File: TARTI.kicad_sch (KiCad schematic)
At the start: 7 parts, among them J1 Conn_01x04_Socket, J2 Conn_01x04_Socket, J3 Screw_Terminal_01x02, U1 LM7805_TO220

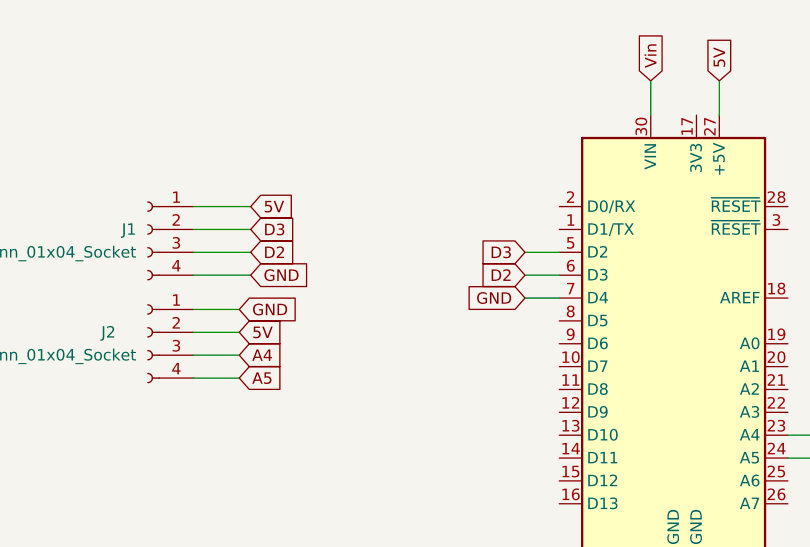
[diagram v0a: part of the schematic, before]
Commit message: Add files via upload
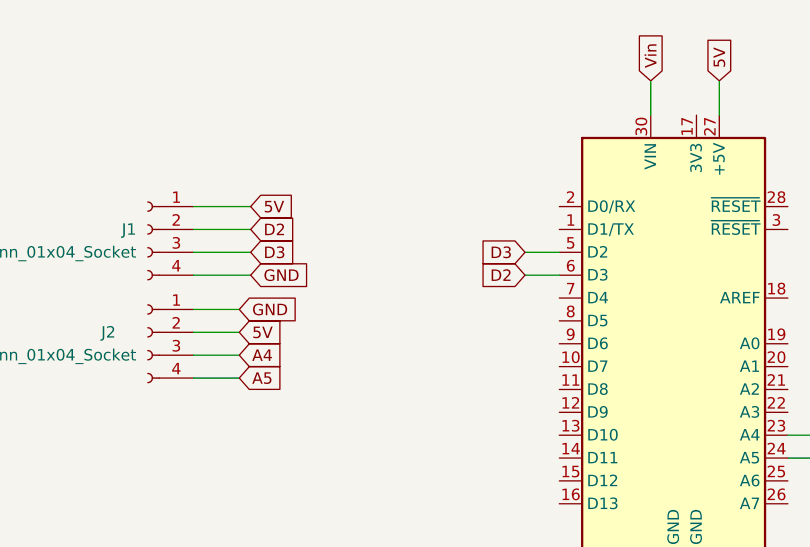
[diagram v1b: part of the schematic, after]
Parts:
- J1, J2: footprint Connector_PinHeader_1.27mm:PinHeader_1x04_P1.27mm_Vertical -> Connector_PinSocket_2.54mm:PinSocket_1x04_P2.54mm_Vertical
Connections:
- net D2: now also J1.2 (Pin_2); no longer J1.3 (Pin_3)
- net D3: now also J1.3 (Pin_3); no longer J1.2 (Pin_2)
- net GND: no longer A1.7 (D4)
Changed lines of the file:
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@@
-		)
-	)
-	(wire
-		(pts
-			(xy 106.68 63.5) (xy 110.49 63.5)
-		)
-		(stroke
-			(width 0)
-			(type default)
 		)
 	)
@@
 		)
 	)
+	(global_label "D2"
+		(shape input)
+		(at 76.2 55.88 0)
+		(fields_autoplaced yes)
+		(effects
+			(font
+				(size 1.27 1.27)
+			)
+			(justify left)
+		)
+		(property "Intersheetrefs" "${INTERSHEET_REFS}"
+			(at 81.6647 55.88 0)
+			(effects
+				(font
+					(size 1.27 1.27)
+				)
+				(justify left)
+				(hide yes)
+			)
+		)
+	)
+	(global_label "GND"
+		(shape input)
+		(at 123.19 97.79 270)
+		(fields_autoplaced yes)
+		(effects
+			(font
+				(size 1.27 1.27)
+			)
+			(justify right)
+		)
+		(property "Intersheetrefs" "${INTERSHEET_REFS}"
+			(at 123.19 104.6457 90)
+			(effects
+				(font
+					(size 1.27 1.27)
+				)
+				(justify right)
+				(hide yes)
+			)
+		)
+	)
+	(global_label "GND"
+		(shape input)
+		(at 49.53 138.43 180)
+		(fields_autoplaced yes)
+		(effects
+			(font
+				(size 1.27 1.27)
+			)
+			(justify right)
+		)
+		(property "Intersheetrefs" "${INTERSHEET_REFS}"
+			(at 42.6743 138.43 0)
+			(effects
+				(font
+					(size 1.27 1.27)
+				)
+				(justify right)
+				(hide yes)
+			)
+		)
+	)
+	(global_label "Vin"
+		(shape input)
+		(at 120.65 39.37 90)
+		(fields_autoplaced yes)
+		(effects
+			(font
+				(size 1.27 1.27)
+			)
+			(justify left)
+		)
+		(property "Intersheetrefs" "${INTERSHEET_REFS}"
+			(at 120.65 33.5424 90)
+			(effects
+				(font
+					(size 1.27 1.27)
+				)
+				(justify left)
+				(hide yes)
+			)
+		)
+	)
 	(global_label "D3"
 		(shape input)
-		(at 76.2 55.88 0)
-		(fields_autoplaced yes)
-		(effects
-			(font
-				(size 1.27 1.27)
-			)
-			(justify left)
-		)
-		(property "Intersheetrefs" "${INTERSHEET_REFS}"
-			(at 81.6647 55.88 0)
-			(effects
-				(font
-					(size 1.27 1.27)
-				)
-				(justify left)
-				(hide yes)
-			)
-		)
-	)
-	(global_label "GND"
-		(shape input)
-		(at 123.19 97.79 270)
+		(at 76.2 58.42 0)
+		(fields_autoplaced yes)
+		(effects
+			(font
+				(size 1.27 1.27)
+			)
+			(justify left)
+		)
+		(property "Intersheetrefs" "${INTERSHEET_REFS}"
+			(at 81.6647 58.42 0)
+			(effects
+				(font
+					(size 1.27 1.27)
+				)
+				(justify left)
+				(hide yes)
+			)
+		)
+	)
+	(global_label "D3"
+		(shape input)
+		(at 106.68 58.42 180)
 		(fields_autoplaced yes)
 		(effects
@@
 		)
 		(property "Intersheetrefs" "${INTERSHEET_REFS}"
-			(at 123.19 104.6457 90)
+			(at 101.2153 58.42 0)
 			(effects
 				(font
@@
 		)
 	)
-	(global_label "GND"
-		(shape input)
-		(at 49.53 138.43 180)
+	(global_label "A5"
+		(shape input)
+		(at 74.93 72.39 0)
+		(fields_autoplaced yes)
+		(effects
+			(font
+				(size 1.27 1.27)
+			)
+			(justify left)
+		)
+		(property "Intersheetrefs" "${INTERSHEET_REFS}"
+			(at 80.2133 72.39 0)
+			(effects
+				(font
+					(size 1.27 1.27)
+				)
+				(justify left)
+				(hide yes)
+			)
+		)
+	)
+	(global_label "Vgiriş"
+		(shape input)
+		(at 46.99 100.33 180)
 		(fields_autoplaced yes)
 		(effects
@@
 		)
 		(property "Intersheetrefs" "${INTERSHEET_REFS}"
-			(at 42.6743 138.43 0)
+			(at 38.7433 100.33 0)
 			(effects
 				(font
@@
 		)
 	)
-	(global_label "Vin"
-		(shape input)
-		(at 120.65 39.37 90)
-		(fields_autoplaced yes)
-		(effects
-			(font
-				(size 1.27 1.27)
-			)
-			(justify left)
-		)
-		(property "Intersheetrefs" "${INTERSHEET_REFS}"
-			(at 120.65 33.5424 90)
-			(effects
-				(font
-					(size 1.27 1.27)
-				)
-				(justify left)
-				(hide yes)
-			)
-		)
-	)
 	(global_label "D2"
 		(shape input)
-		(at 76.2 58.42 0)
-		(fields_autoplaced yes)
-		(effects
-			(font
-				(size 1.27 1.27)
-			)
-			(justify left)
-		)
-		(property "Intersheetrefs" "${INTERSHEET_REFS}"
-			(at 81.6647 58.42 0)
-			(effects
-				(font
-					(size 1.27 1.27)
-				)
-				(justify left)
-				(hide yes)
-			)
-		)
-	)
-	(global_label "D3"
-		(shape input)
-		(at 106.68 58.42 180)
+		(at 106.68 60.96 180)
 		(fields_autoplaced yes)
 		(effects
@@
 		)
 		(property "Intersheetrefs" "${INTERSHEET_REFS}"
-			(at 101.2153 58.42 0)
-			(effects
-				(font
-					(size 1.27 1.27)
-				)
-				(justify right)
-				(hide yes)
-			)
-		)
-	)
-	(global_label "A5"
-		(shape input)
-		(at 74.93 72.39 0)
-		(fields_autoplaced yes)
-		(effects
-			(font
-				(size 1.27 1.27)
-			)
-			(justify left)
-		)
-		(property "Intersheetrefs" "${INTERSHEET_REFS}"
-			(at 80.2133 72.39 0)
-			(effects
-				(font
-					(size 1.27 1.27)
-				)
-				(justify left)
-				(hide yes)
-			)
-		)
-	)
-	(global_label "Vgiriş"
-		(shape input)
-		(at 46.99 100.33 180)
-		(fields_autoplaced yes)
-		(effects
-			(font
-				(size 1.27 1.27)
-			)
-			(justify right)
-		)
-		(property "Intersheetrefs" "${INTERSHEET_REFS}"
-			(at 38.7433 100.33 0)
-			(effects
-				(font
-					(size 1.27 1.27)
-				)
-				(justify right)
-				(hide yes)
-			)
-		)
-	)
-	(global_label "D2"
-		(shape input)
-		(at 106.68 60.96 180)
-		(fields_autoplaced yes)
-		(effects
-			(font
-				(size 1.27 1.27)
-			)
-			(justify right)
-		)
-		(property "Intersheetrefs" "${INTERSHEET_REFS}"
 			(at 101.2153 60.96 0)
-			(effects
-				(font
-					(size 1.27 1.27)
-				)
-				(justify right)
-				(hide yes)
-			)
-		)
-	)
-	(global_label "GND"
-		(shape input)
-		(at 106.68 63.5 180)
-		(fields_autoplaced yes)
-		(effects
-			(font
-				(size 1.27 1.27)
-			)
-			(justify right)
-		)
-		(property "Intersheetrefs" "${INTERSHEET_REFS}"
-			(at 99.8243 63.5 0)
 			(effects
 				(font
@@
 			)
 		)
-		(property "Footprint" "Connector_PinHeader_1.27mm:PinHeader_1x04_P1.27mm_Vertical"
+		(property "Footprint" "Connector_PinSocket_2.54mm:PinSocket_1x04_P2.54mm_Vertical"
 			(at 64.77 67.31 0)
 			(effects
@@
 			)
 		)
-		(property "Footprint" "Connector_PinHeader_1.27mm:PinHeader_1x04_P1.27mm_Vertical"
+		(property "Footprint" "Connector_PinSocket_2.54mm:PinSocket_1x04_P2.54mm_Vertical"
 			(at 64.77 55.88 0)
 			(effects
